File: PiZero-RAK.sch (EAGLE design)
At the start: 22 parts, among them J1 2.54_I2C, J11 CON_HEADER_1X06-PTH, J2 CONN_20X2HLE, J7 2.54_I2C, J9 2.54_I2C, X1 SPTAF_23.5, X2 SPTAF_25.0MM

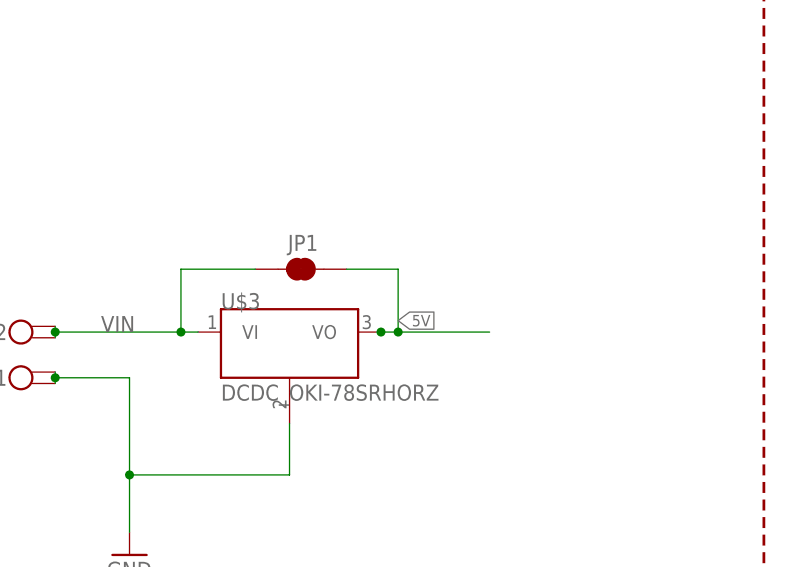
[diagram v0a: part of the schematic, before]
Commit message: Bump to V1.3b
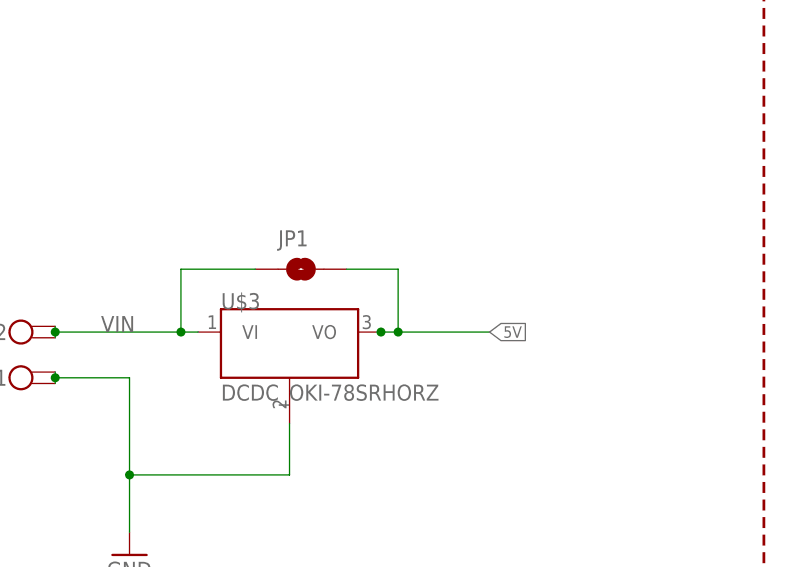
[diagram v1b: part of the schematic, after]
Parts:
- JP1: value 5VIN -> JUMPER-PAD-2-NOYES_SILK; device SparkFun-Passives:JUMPER-PAD-2-NC_BY_TRACE -> SparkFun-Passives:JUMPER-PAD-2-NOYES_SILK
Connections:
- net 5V: now also JP1.2; no longer JP1.1
- net VIN: now also JP1.1; no longer JP1.2
